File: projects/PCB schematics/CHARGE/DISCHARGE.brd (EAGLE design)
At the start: 99.1 x 99.1 mm, 11 parts

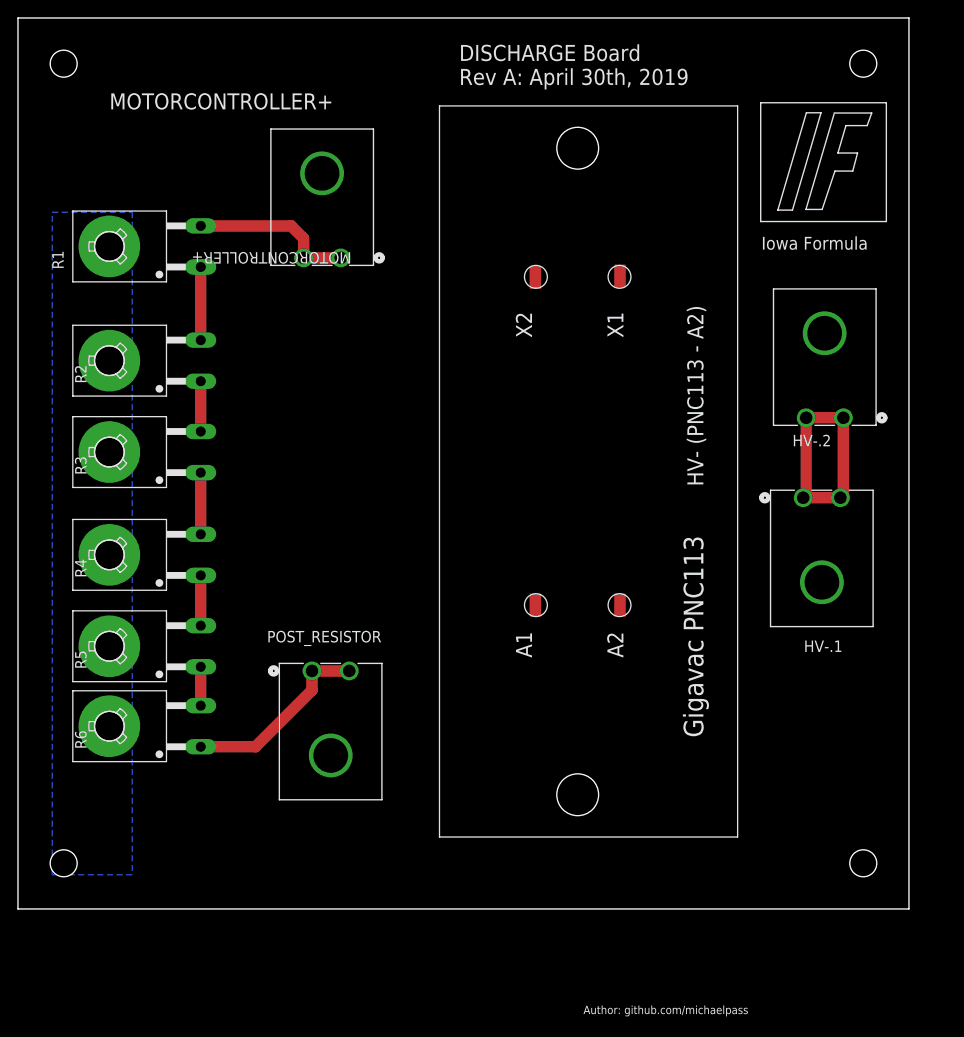
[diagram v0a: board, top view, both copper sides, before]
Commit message: PROJ - Final pre-purchase revisions (4 boards still in progress.)
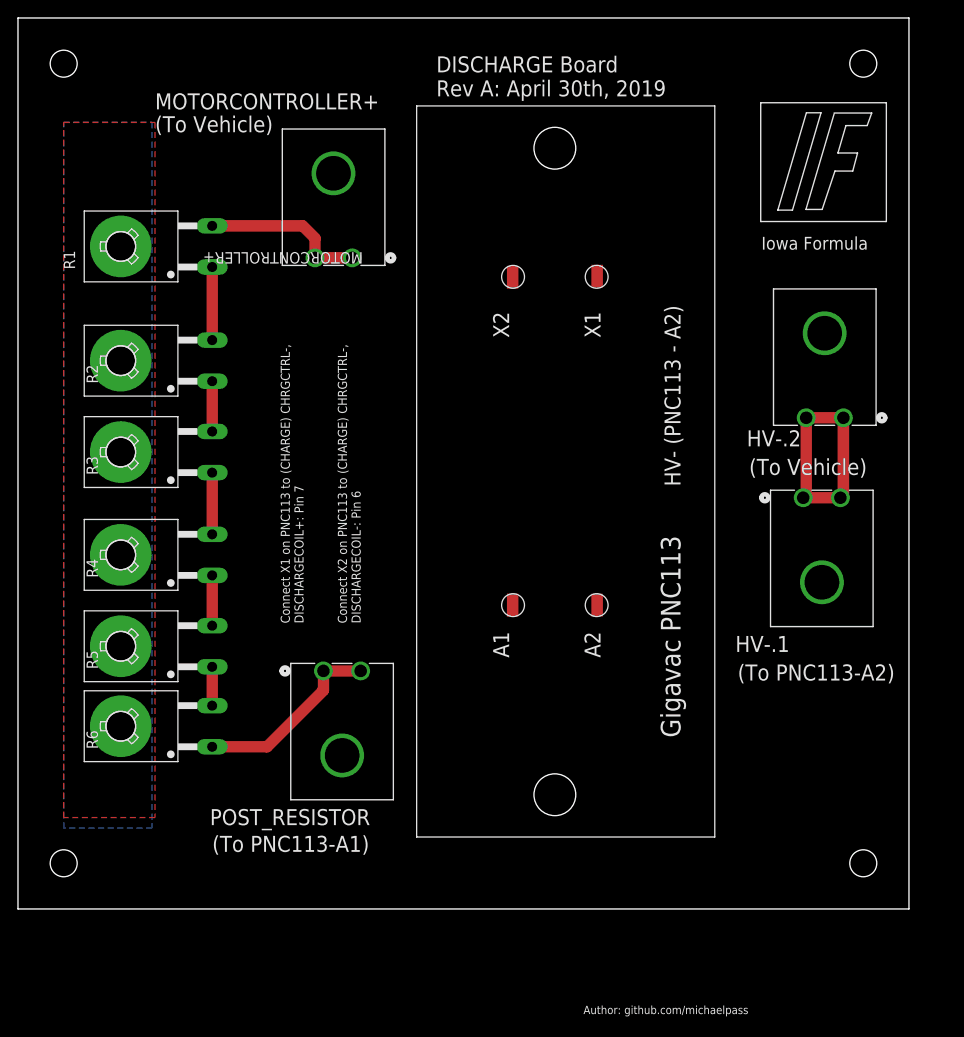
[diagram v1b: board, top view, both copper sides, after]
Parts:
- moved PNC113 2.54 mm to (59.7, 12.7)
- moved MOTORCONTROLLER+ 1.27 mm to (33.0, 72.4)
- moved POST_RESISTOR 1.27 mm to (38.1, 26.5)
- moved R1 1.27 mm to (16.5, 73.7)
- moved R2 1.27 mm to (16.5, 61.0)
- moved R3 1.27 mm to (16.5, 50.8)
- moved R4 1.27 mm to (16.5, 39.4)
- moved R5 1.27 mm to (16.5, 29.2)
- moved R6 1.27 mm to (16.5, 20.3)
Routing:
- added copper zone on layer 1, net HEATSINK
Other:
- board text added: "(To PNC113-A1)"
- board text added: "(To PNC113-A2)"
- board text added: "(To Vehicle)"
- board text added: "Connect X1 on PNC113 to (CHARGE) CHRGCTRL-, DISCHARGECOIL+: Pin 7"
- board text added: "Connect X2 on PNC113 to (CHARGE) CHRGCTRL-, DISCHARGECOIL-: Pin 6"
